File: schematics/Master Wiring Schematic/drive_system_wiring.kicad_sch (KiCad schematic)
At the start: 8 parts, among them J10 Front Left Motor, J11 Left_BTS7960_Logic, J12 Right_BTS7960_Logic, J5 Rear Left Motor, J6 Left_BTS7960_PWR, J7 Right_BTS7960_PWR, J8 Front Right Motor, J9 Rear Right Motor

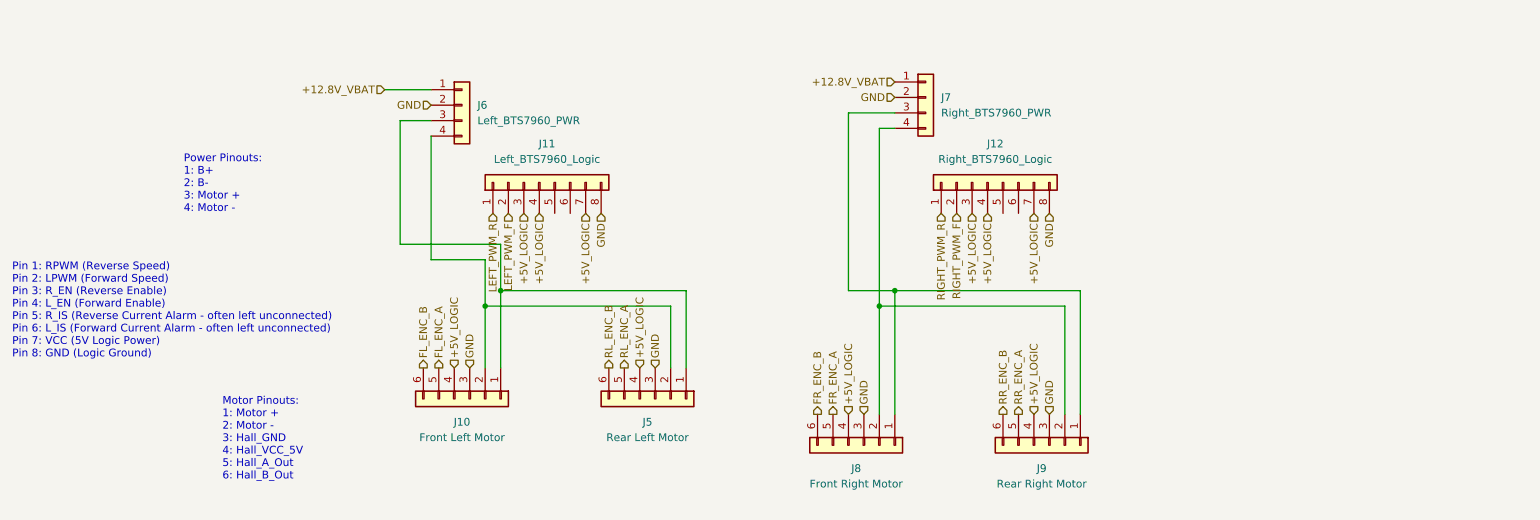
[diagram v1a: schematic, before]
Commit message: Aesthetification of V1
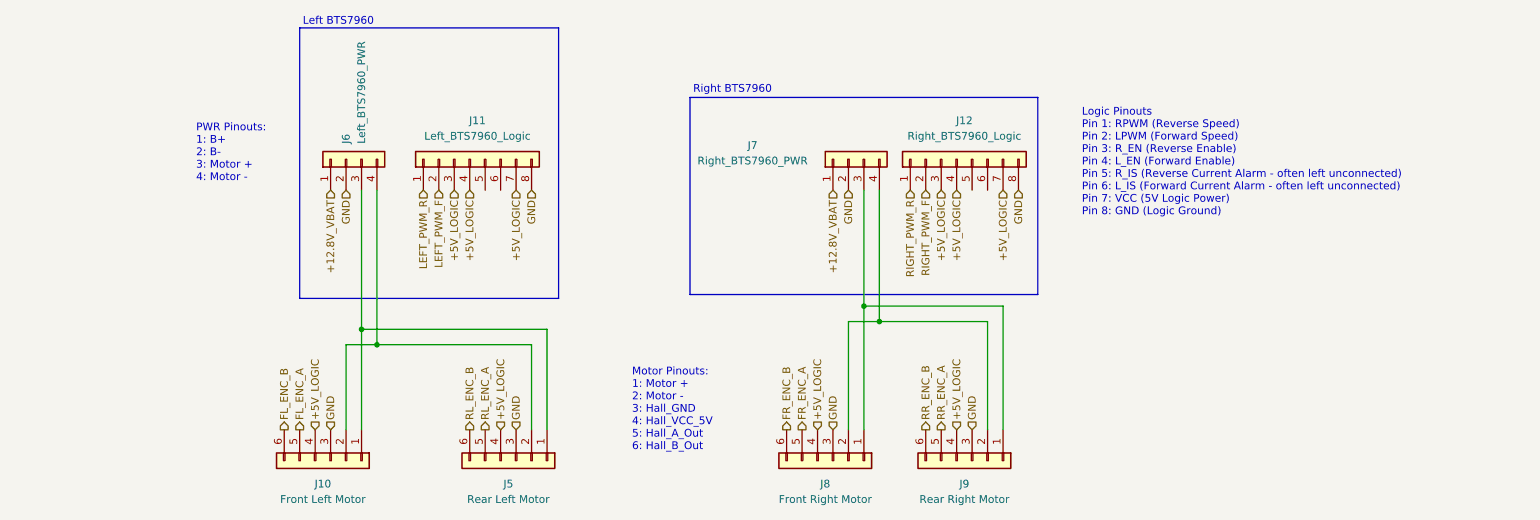
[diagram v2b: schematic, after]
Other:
- note added: "Left BTS7960"
- note added: "Logic Pinouts Pin 1: RPWM (Reverse Speed) Pin 2: LPWM (Forward Speed) Pin 3: R_EN (Reverse Enable) Pin 4: L_EN (Forward Enable) Pin 5: R_IS (Reverse Current Alarm - often left unconnected) Pin 6: L_IS (Forward Current Alarm - often left unconnected) Pin 7: VCC (5V Logic Power) Pin 8: GND (Logic Ground)"
- note added: "PWR Pinouts: 1: B+ 2: B- 3: Motor + 4: Motor -"
- note added: "Right BTS7960"
- note removed: "Pin 1: RPWM (Reverse Speed) Pin 2: LPWM (Forward Speed) Pin 3: R_EN (Reverse Enable) Pin 4: L_EN (Forward Enable) Pin 5: R_IS (Reverse Current Alarm - often left unconnected) Pin 6: L_IS (Forward Current Alarm - often left unconnected) Pin 7: VCC (5V Logic Power) Pin 8: GND (Logic Ground)"
- note removed: "Power Pinouts: 1: B+ 2: B- 3: Motor + 4: Motor -"
- moved on the sheet: J10, J11, J12, J5, J6, J7, J8, J9
